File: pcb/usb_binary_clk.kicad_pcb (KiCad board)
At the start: 2 copper layers, 40 parts, among them J1 USB_B_Micro, J2 USB_B_Micro, SW1 SW_Push, SW2 SW_Push, SW3 SW_Push, U1 MCP7940N-xP, U2 ATtiny84V-10PU, Y1 Crystal

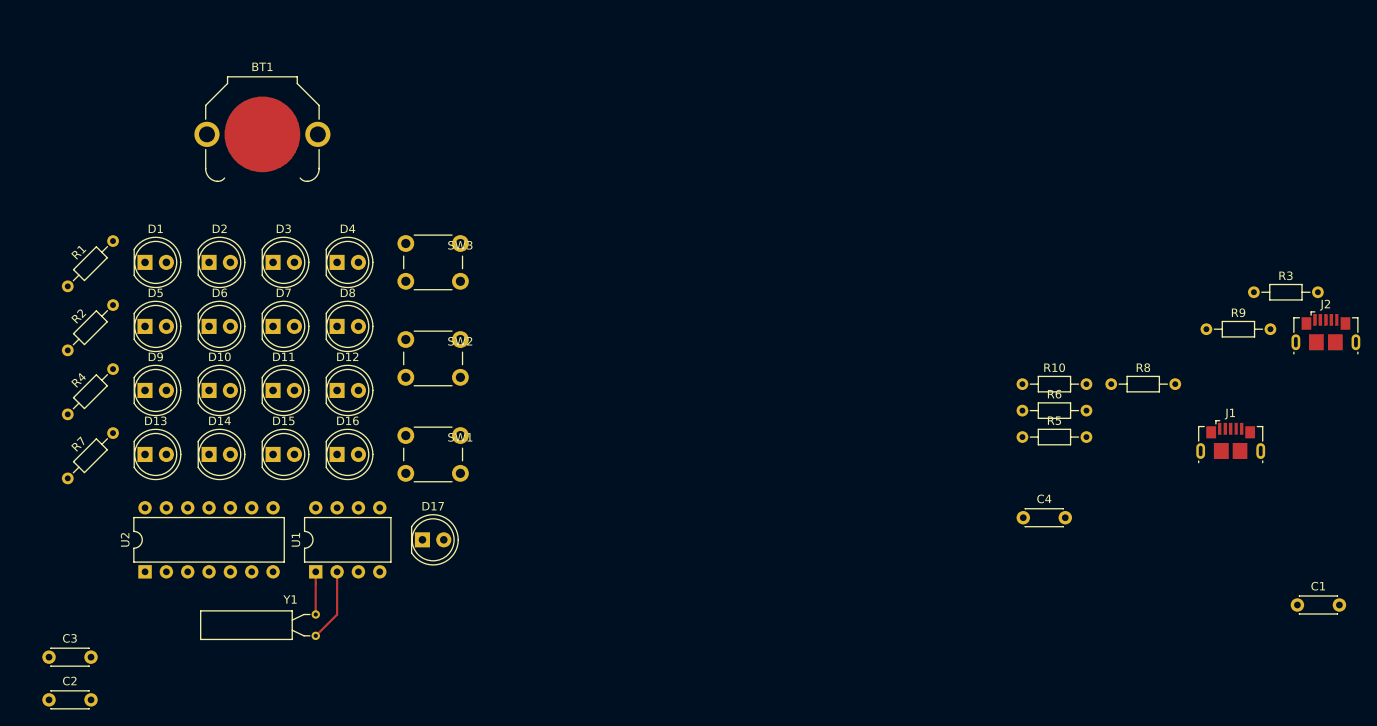
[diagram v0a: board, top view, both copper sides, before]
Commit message: Modify pcb layout
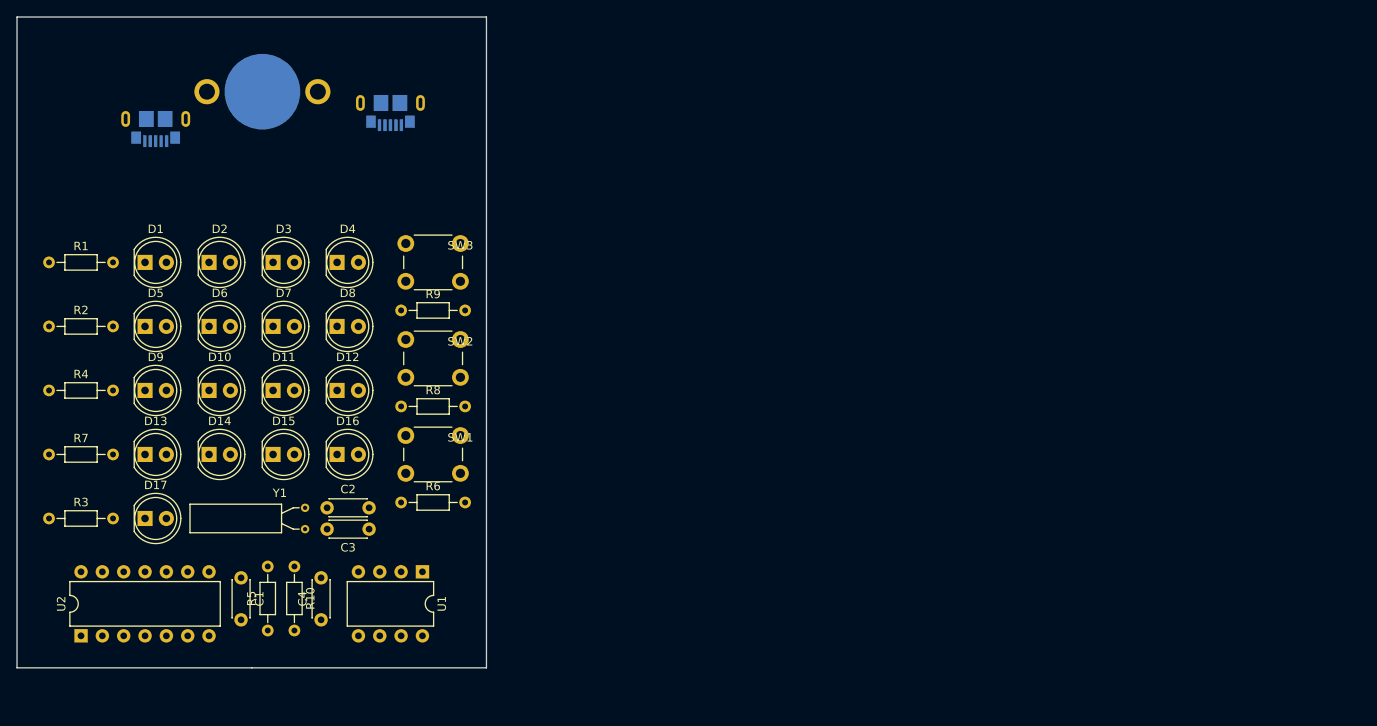
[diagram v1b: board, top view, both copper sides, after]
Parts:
- BT1, J1, J2: moved to B.Cu
- moved R3 145.9 mm to (129.5, 76.2)
- moved J1 133.2 mm to (142.2, 29.8)
- moved C1 125.8 mm to (152.4, 83.3), turned to 270 degrees
- moved J2 114.4 mm to (170.2, 27.9)
- moved R9 95.9 mm to (171.4, 51.4)
- moved R5 92.7 mm to (155.6, 89.5), turned to 90 degrees
- moved R10 89.3 mm to (158.8, 81.9), turned to 270 degrees
- moved R8 84.6 mm to (171.4, 62.9)
- moved C4 84.5 mm to (161.9, 88.3), turned to 90 degrees
- moved R6 74.8 mm to (171.4, 74.3)
- moved C3 41.0 mm to (167.6, 77.5), turned to 180 degrees
- moved C2 40.2 mm to (162.6, 74.9)
- moved D17 33.1 mm to (142.2, 76.2)
- moved Y1 12.8 mm to (160.0, 74.9)
- moved U1 12.7 mm to (174.0, 82.5), turned to 270 degrees
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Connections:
- U1 pad 5: /scl -> /sda
- U1 pad 6: /sda -> /scl
- Y1 pad 1: /clk- -> /clk+
- Y1 pad 2: /clk+ -> /clk-
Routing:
- net /clk+: track 8.67 -> 0.11 mm
- net /clk-: track 5.08 -> 0.00 mm
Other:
- board outline added: 55.9 x 77.5 mm
